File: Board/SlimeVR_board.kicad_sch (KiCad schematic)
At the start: 36 parts, among them IC1 HT7833, J1 USB_C_Receptacle_USB2.0_16P, J2 JST-PH, J3 SMD_Pads, J5 Conn_01x01_Pin, J6 Conn_01x01_Pin, J7 JTX-HX, Q1 DMP3099L-7, SW1 LA215009, U1 TP4056-42-ESOP8, U2 ESP32-C3-WROOM-02

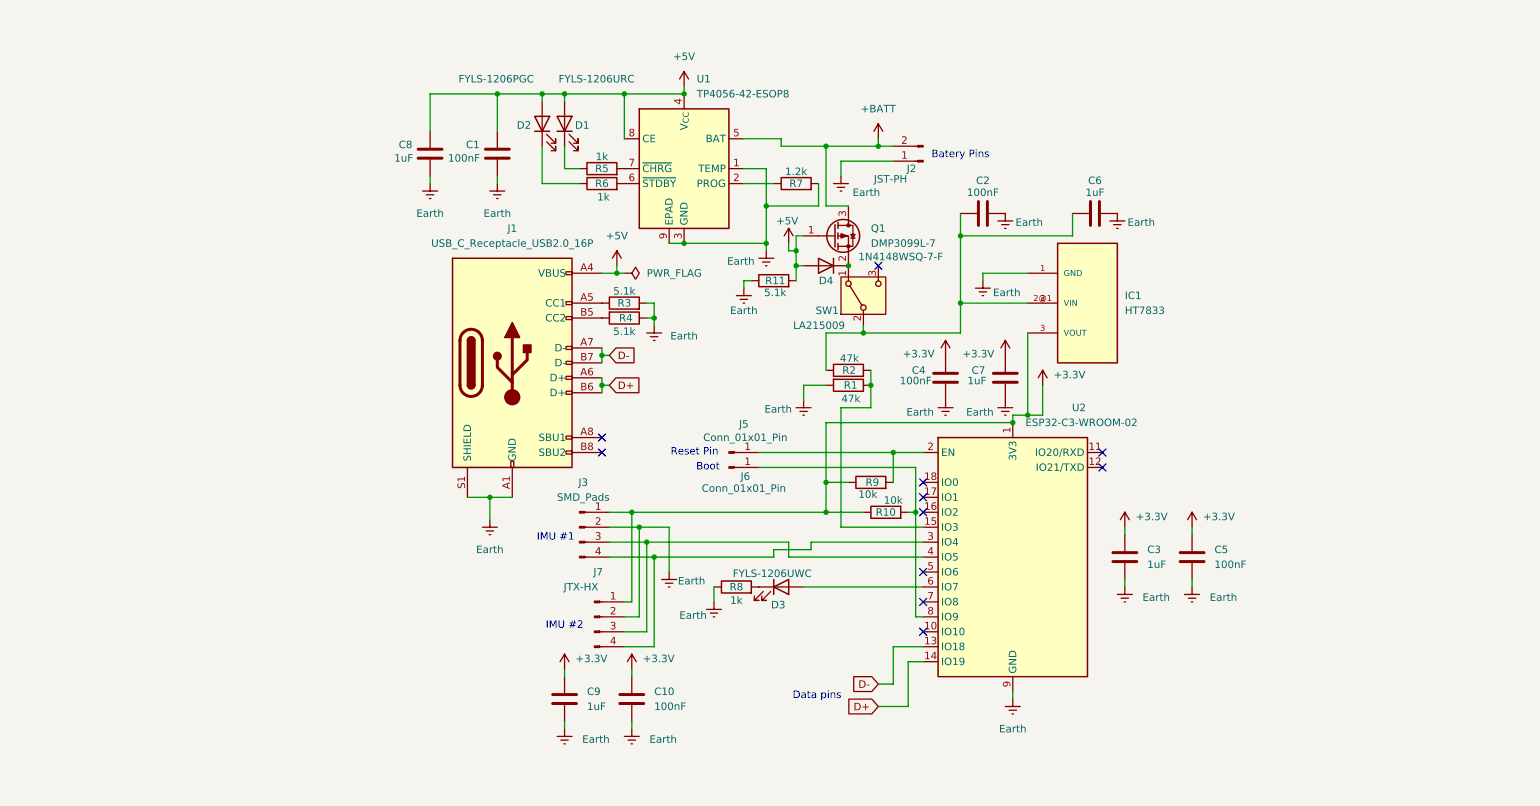
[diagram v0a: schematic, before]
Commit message: New version
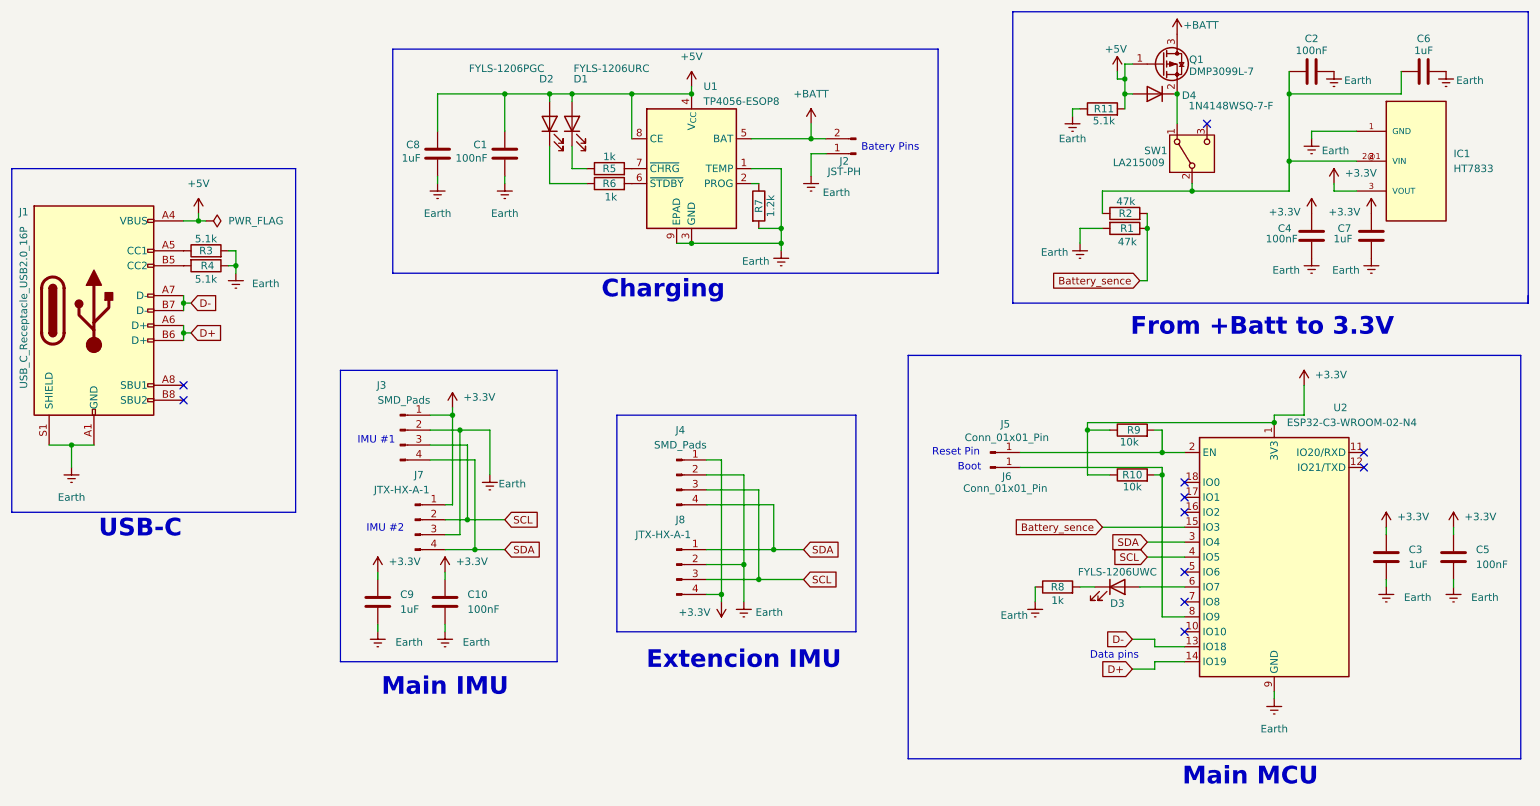
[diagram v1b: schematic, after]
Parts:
- added J4: SMD_Pads, Custom:Pin_1x04_SMD_P2.54mm, symbol Connector:Conn_01x04_Pin
- added J8: JTX-HX-A-1, Connector_JST:JST_XH_S4B-XH-A-1_1x04_P2.50mm_Horizontal, symbol Connector:Conn_01x04_Pin
- J7: value JTX-HX -> JTX-HX-A-1; footprint Connector_JST:JST_XH_S4B-XH-A_1x04_P2.50mm_Horizontal -> Connector_JST:JST_XH_S4B-XH-A-1_1x04_P2.50mm_Horizontal
- U1: value TP4056-42-ESOP8 -> TP4056-ESOP8
- U2: value ESP32-C3-WROOM-02 -> ESP32-C3-WROOM-02-N4
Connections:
- net +3.3V: now also J4.1 (Pin_1), J8.4 (Pin_4)
- net Earth: now also J7.3 (Pin_3), J4.2 (Pin_2), J8.2 (Pin_2); no longer J7.2 (Pin_2)
- net Battery_sence: now reaches R1.1, R2.2, U2.15 (IO3)
- net SCL: now reaches J3.3 (Pin_3), U2.4 (IO5)
- net SCL: now also J7.2 (Pin_2), J4.3 (Pin_3), J8.3 (Pin_3); no longer J7.3 (Pin_3)
- net SDA: now reaches J3.4 (Pin_4), J7.4 (Pin_4), U2.3 (IO4)
- net SDA: now also J4.4 (Pin_4), J8.1 (Pin_1)
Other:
- note added: "Charging"
- note added: "Extencion IMU"
- note added: "From +Batt to 3.3V"
- note added: "Main IMU"
- note added: "Main MCU"
- note added: "USB-C"
- moved on the sheet: C1, C10, C2, C3, C4, C5, C6, C7, C8, C9, D1, D2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
